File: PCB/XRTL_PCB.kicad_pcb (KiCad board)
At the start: 2 copper layers, 94 x 78.7 mm, 20 parts, among them J1 POWER, J10 servo1, J11 servo2, J12 infoLED, J2 stepper1, J3 stepper2, J4 ESP32 right, J5 ESP32 left, J6 relay1 IN, J7 relay2 IN, J8 relay1 OUT, J9 relay2 OUT, K1 TIANBO-HJR-4102-L, K2 TIANBO-HJR-4102-L, U1 TBD62003, U2 TBD62003

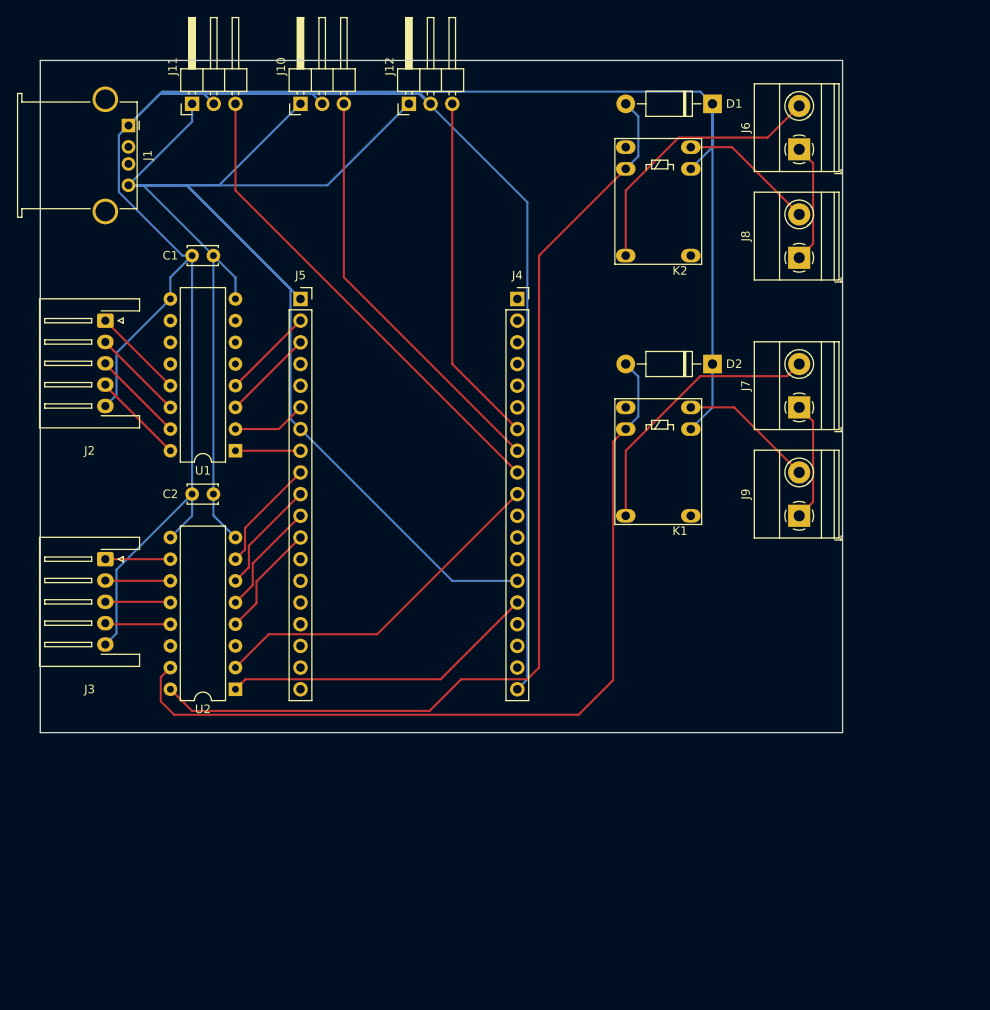
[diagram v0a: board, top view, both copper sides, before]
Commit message: Add files via upload
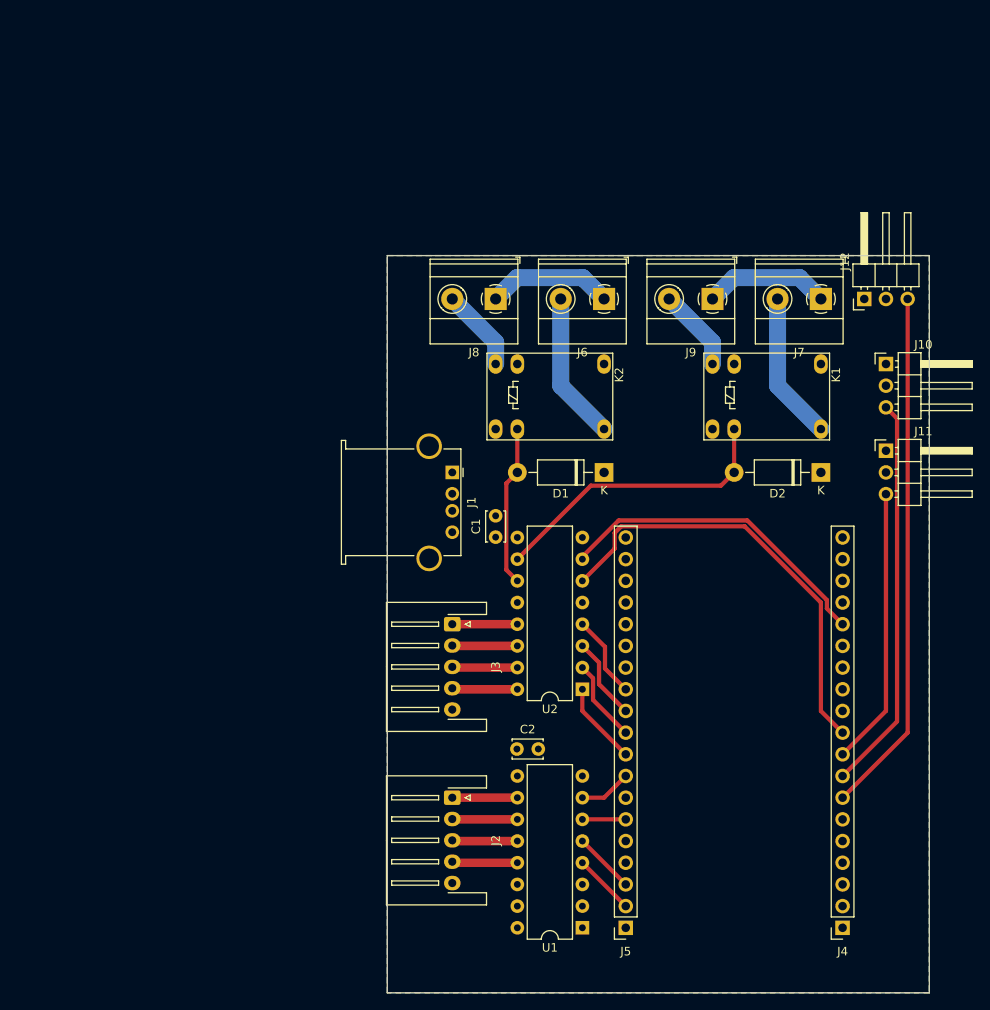
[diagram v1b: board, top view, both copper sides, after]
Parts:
- J6: value relay1 IN -> relay2 IN
- J7: value relay2 IN -> relay1 IN
- J8: value relay1 OUT -> relay2 OUT
- J9: value relay2 OUT -> relay1 OUT
- moved J11 90.9 mm to (132.1, 71.1), turned to 0 degrees
- moved J4 82.9 mm to (127.0, 127.0), turned to 180 degrees
- moved J5 82.9 mm to (101.6, 127.0), turned to 180 degrees
- moved J10 75.0 mm to (132.1, 61.0), turned to 0 degrees
- moved J2 69.1 mm to (81.3, 111.8)
- moved U1 69.1 mm to (96.5, 127.0)
- moved J12 58.0 mm to (129.5, 53.3)
- moved J1 55.6 mm to (81.3, 73.7)
- moved C1 48.5 mm to (86.4, 81.2), turned to 90 degrees
- moved C2 48.4 mm to (88.9, 106.1)
- moved D1 45.0 mm to (99.1, 73.7)
- moved J3 41.3 mm to (81.3, 91.4)
- moved U2 40.6 mm to (96.5, 99.1)
- moved J8 35.9 mm to (86.4, 53.3), turned to 180 degrees
- moved J6 28.8 mm to (99.1, 53.3), turned to 180 degrees
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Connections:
- D1 pad 2: driverRelay1 -> driverRelay2
- D2 pad 2: driverRelay2 -> driverRelay1
- J2 pad 1: Net-(U1-Pad13) -> Net-(J2-Pad1)
- J2 pad 2: Net-(U1-Pad14) -> Net-(J2-Pad2)
- J2 pad 3: Net-(U1-Pad15) -> Net-(U1-Pad12)
- J2 pad 4: Net-(U1-Pad16) -> Net-(U1-Pad13)
- J3 pad 1: Net-(U2-Pad10) -> Net-(J3-Pad1)
- J3 pad 2: Net-(U2-Pad11) -> Net-(J3-Pad2)
- J3 pad 3: Net-(U2-Pad12) -> Net-(J3-Pad3)
- J3 pad 4: Net-(U2-Pad13) -> Net-(U2-Pad16)
- J5 pad 10: stepper2B -> stepper2C
- J5 pad 11: stepper2C -> stepper2B
- J5 pad 12: stepper2D -> stepper2A
- J5 pad 2: stepper1A -> stepper1D
- J5 pad 3: stepper1B -> stepper1C
- J5 pad 6: stepper1C -> stepper1B
- J5 pad 8: stepper1D -> stepper1A
- J5 pad 9: stepper2A -> stepper2D
- K1 pad 8: driverRelay2 -> driverRelay1
- K2 pad 8: driverRelay1 -> driverRelay2
- U1 pad 1: stepper1D -> unconnected-(U1-Pad1)
- U1 pad 10: unconnected-(U1-Pad10) -> Net-(J2-Pad1)
- U1 pad 11: unconnected-(U1-Pad11) -> Net-(J2-Pad2)
- U1 pad 12: unconnected-(U1-Pad12) -> Net-(U1-Pad12)
- U1 pad 14: Net-(U1-Pad14) -> unconnected-(U1-Pad14)
- U1 pad 15: Net-(U1-Pad15) -> unconnected-(U1-Pad15)
- U1 pad 16: Net-(U1-Pad16) -> unconnected-(U1-Pad16)
- U1 pad 2: stepper1C -> unconnected-(U1-Pad2)
- U1 pad 3: stepper1B -> unconnected-(U1-Pad3)
- U1 pad 4: stepper1A -> stepper1D
- U1 pad 5: unconnected-(U1-Pad5) -> stepper1C
- U1 pad 6: unconnected-(U1-Pad6) -> stepper1B
- U1 pad 7: unconnected-(U1-Pad7) -> stepper1A
- U2 pad 1: relay1 -> stepper2D
- U2 pad 10: Net-(U2-Pad10) -> driverRelay1
- U2 pad 11: Net-(U2-Pad11) -> driverRelay2
- U2 pad 12: Net-(U2-Pad12) -> unconnected-(U2-Pad12)
- U2 pad 13: Net-(U2-Pad13) -> Net-(J3-Pad1)
- U2 pad 14: unconnected-(U2-Pad14) -> Net-(J3-Pad2)
- U2 pad 15: driverRelay2 -> Net-(J3-Pad3)
- U2 pad 16: driverRelay1 -> Net-(U2-Pad16)
- U2 pad 2: relay2 -> stepper2C
- U2 pad 3: unconnected-(U2-Pad3) -> stepper2B
- U2 pad 4: stepper2D -> stepper2A
- U2 pad 5: stepper2C -> unconnected-(U2-Pad5)
- U2 pad 6: stepper2B -> relay2
- U2 pad 7: stepper2A -> relay1
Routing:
- net +5V: track 385.6 -> 0.00 mm
- net GND: track 219.7 -> 0.00 mm
- net driverRelay1: track 117.8 -> 34.7 mm
- net driverRelay2: track 98.6 -> 18.8 mm
- net servo2: track 56.9 -> 32.6 mm
- net infoLED: track 41.3 -> 61.6 mm
- net Net-(J7-Pad2): track 32.1 -> 17.3 mm
- net Net-(J6-Pad2): track 32.0 -> 17.3 mm
- net Net-(U1-Pad16): track 10.9 -> 0.00 mm
- net Net-(U1-Pad15): track 10.9 -> 0.00 mm
- net Net-(U1-Pad14): track 10.8 -> 0.00 mm
- net relay2: track 41.4 -> 51.6 mm
- net Net-(J3-Pad3): track 0.00 -> 7.73 mm
- net Net-(J3-Pad2): track 0.00 -> 7.69 mm
- net Net-(J2-Pad2): track 0.00 -> 7.69 mm
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- added copper zone on F.Cu, net +5V
- added copper zone on B.Cu, net GND
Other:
- board size 94 x 78.7 mm -> 63.5 x 86.4 mm
